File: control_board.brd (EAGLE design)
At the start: 90.2 x 72.3 mm, 19 parts

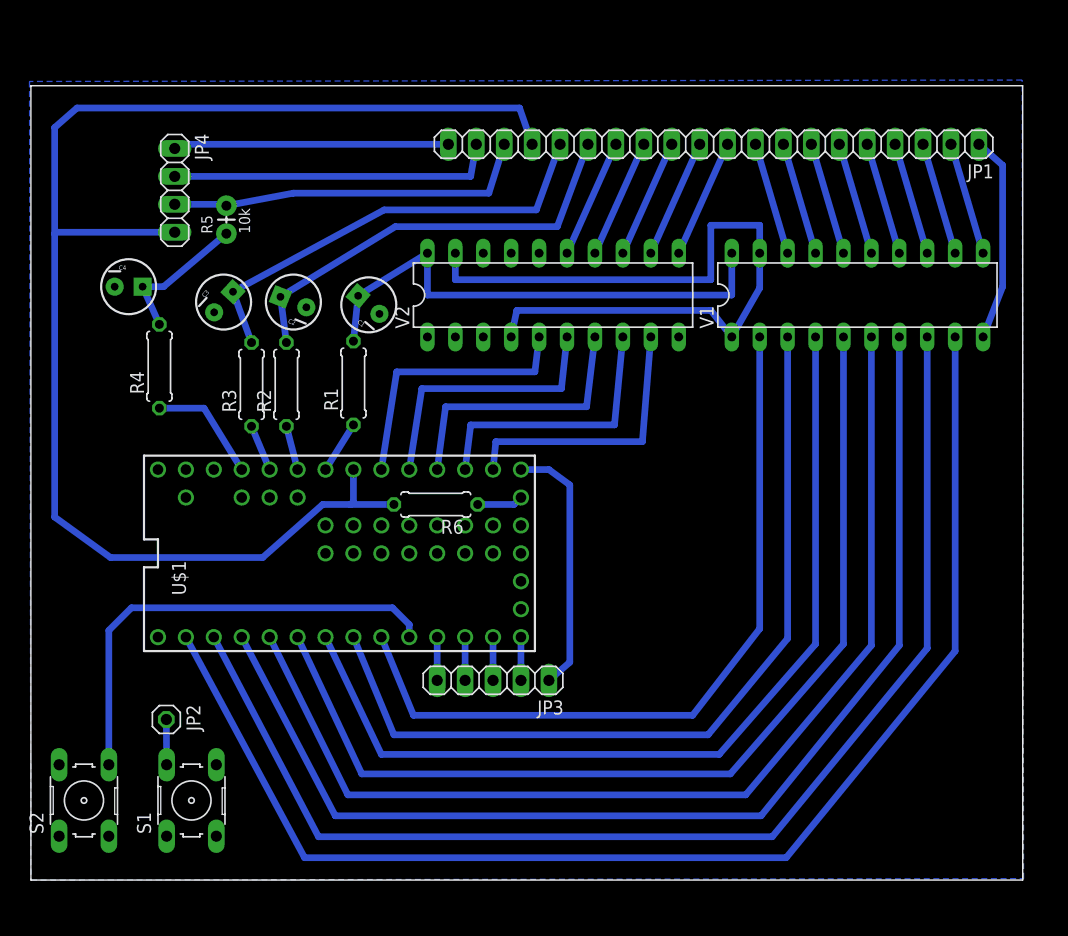
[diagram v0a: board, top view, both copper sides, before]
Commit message: First commit
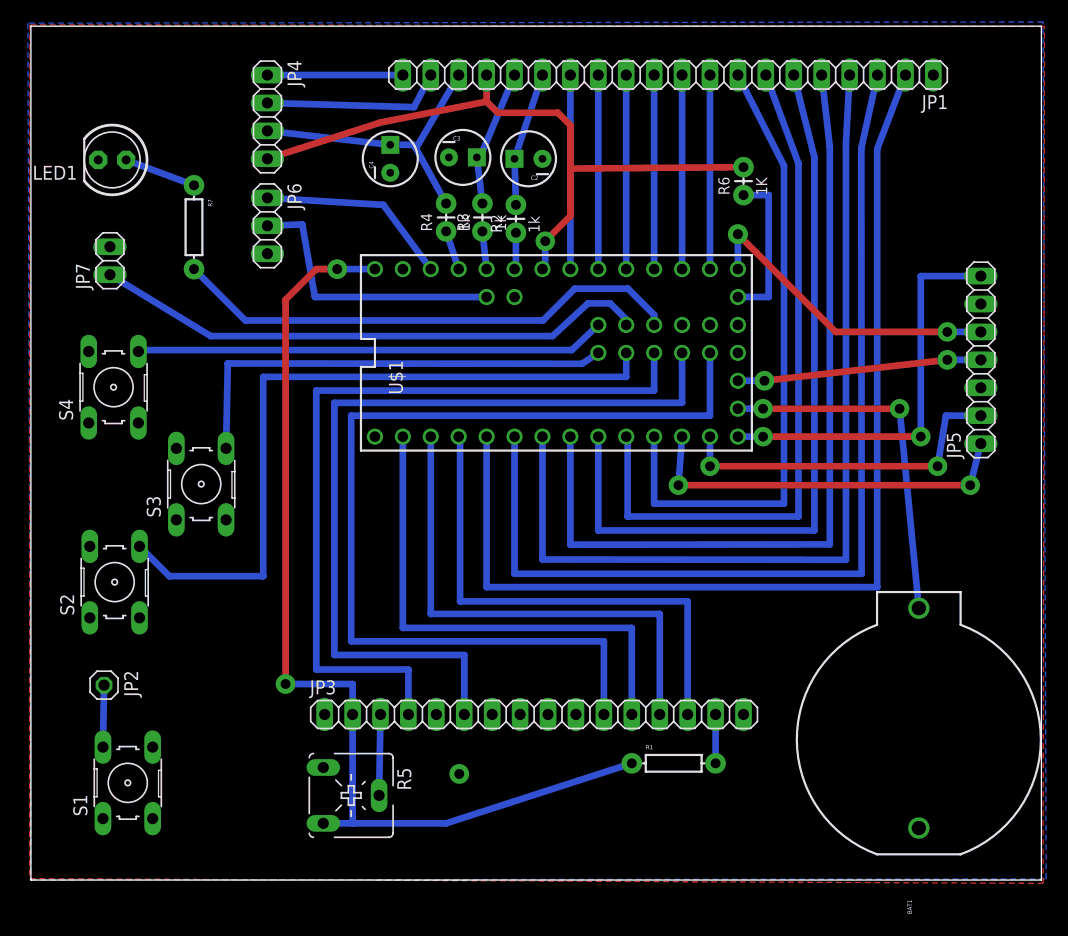
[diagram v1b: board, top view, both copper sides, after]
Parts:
- removed C1: (no value), SparkFun-Capacitors:CPOL-RADIAL-10UF-25V
- removed V1, V2: 74540N, 74ttl-din:DIL20
- added BAT1: (no value), SparkFun-Electromechanical:BATTCOM_20MM_PTH
- added JP5: SD_card, sd_header:1X07
- added JP6: (no value), pinhead:1X03
- added JP7: Buzzer_header, pinhead:1X02
- added LED1: (no value), adafruit:LED5MM
- added R7: (no value), SparkFun-Resistors:AXIAL-0.3EZ
- added S3, S4: (no value), switch-omron:B3F-10XX
- JP3: value (none) -> 16x2_LCD_header; device pinhead:1X05 -> LCD_HEADER:1X16
- R1: value 330 -> (none); device resistor:0207/7 -> SparkFun-Resistors:AXIAL-0.3EZ
- R2, R3, R4: device resistor:0207/7 -> SparkFun-Resistors:AXIAL-0.1
- R5: value 10k -> (none); device SparkFun-Resistors:AXIAL-0.1 -> pot:CA6V
- R6: device rcl:0207/7 -> SparkFun-Resistors:AXIAL-0.1
- U$1: value TEENSY_3.0_ALLPINS -> TEENSY_31_ALLPINS_DIGITAL; device Teensy3.0:TEENSY_3.0_ALLPINS -> Teensy3.0:TEENSY_31_ALLPINS_DIGITAL
- moved R5 52.4 mm to (29.1, 7.70), turned to 270 degrees
- moved R1 45.2 mm to (58.5, 10.6), turned to 0 degrees
- moved R6 39.7 mm to (64.8, 62.3), turned to 90 degrees
- moved R4 28.8 mm to (37.8, 59.0)
- moved U$1 27.8 mm to (49.1, 48.0)
- moved C4 26.5 mm to (32.7, 65.6), turned to 90 degrees
- moved C3 25.4 mm to (39.3, 65.7), turned to 0 degrees
- moved R3 25.2 mm to (41.1, 59.0)
- moved C2 25.0 mm to (45.3, 65.6), turned to 180 degrees
- moved R2 25.0 mm to (44.1, 58.9)
- moved S2 20.1 mm to (7.62, 27.1)
- moved JP4 10.8 mm to (21.5, 69.4)
- moved JP1 7.54 mm to (58.0, 73.2)
- moved JP2 6.47 mm to (6.65, 17.7)
- moved S1 6.01 mm to (8.81, 8.84)
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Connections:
- removed net +UB: C1.1, R1.2, V1.20, V2.20
- removed net AREF: U$1.AREF
- removed net LEVEL_SHIFTER_POWER_PIN: R1.1, U$1.20/A6
- removed net N0: C4.1, R4.2, R5.P$1
- removed net VBAT: U$1.VBAT
- removed net VIN: U$1.VIN
- removed net VUSB: U$1.VUSB
- new net 3.3V: JP5.3V3, JP6.1, U$1.3.3V
- new net N$37: JP7.1, U$1.32
- net 3DS_C_PAD_X: now also R2.P$2; no longer R2.2
- net 3DS_C_PAD_Y: now also R3.P$2; no longer R3.2
- net 3DS_TOUCH_SCREEN_X: now also C4.1, R4.P$2; no longer R5.P$2
- net 3DS_TOUCH_SCREEN_Y: now also R6.P$2, U$1.20/A6; no longer R6.2, U$1.19/A5
- net C_PAD_X_PIN: now also R2.P$1; no longer R2.1
- net C_PAD_Y_PIN: now also R3.P$1; no longer R3.1
- net GND: now also BAT1.2, JP3.GND, JP3.LED-, JP3.RW, JP5.GND, JP5.GND_2, JP6.3, JP7.2, LED1.K, R5.A, S3.2, S4.2; no longer C1.2, U$1.GND1, U$1.GND2, V1.1, V1.10, V1.19, V2.1, V2.10, V2.19, V2.2, V2.3, V2.4
- net N$1: now also JP1.7, U$1.8; no longer JP1.2, V1.11
- net N$10: now also JP3.CONTRAST, R5.S; no longer JP1.12, V2.13
- net N$11: now also JP5.SS, U$1.10; no longer JP1.13, V2.14
- net N$12: now also JP5.MOSI, U$1.11; no longer JP1.14, V2.15
- net N$13: now also JP5.MISO, U$1.12; no longer JP1.10, V2.11
- net N$15: now also JP5.SCK, U$1.13; no longer U$1.14/A0, V2.9
- net N$16: now also JP6.2, U$1.A10; no longer U$1.15/A1, V2.8
- net N$17: now also JP3.D7, U$1.2; no longer U$1.16/A2, V2.7
- net N$18: now also JP3.D6, U$1.1; no longer U$1.17/A3, V2.6
- net N$19: now also JP3.D5; no longer V1.9
- net N$2: now also JP1.8, U$1.9; no longer JP1.3, V1.12
- net N$20: now also JP3.D4, U$1.28; no longer U$1.1, V1.8
- net N$21: now also JP3.E, U$1.27; no longer U$1.2, V1.7
- net N$22: now also JP1.2; no longer V1.6
- net N$23: now also JP1.3; no longer V1.5
- net N$24: now also JP1.4; no longer V1.4
- net N$25: now also JP1.5; no longer V1.3
- net N$26: now also JP1.6; no longer V1.2
- net N$27: now also R6.P$1; no longer R6.1
- net N$28: now also JP3.RS, U$1.26; no longer U$1.18/A4, V2.5
- net N$29: now also BAT1.1, U$1.VBAT; no longer JP3.5, U$1.9
- net N$3: now also JP1.9, U$1.14/A0; no longer JP1.4, V1.13
- net N$30: now also S2.4, U$1.25; no longer JP3.4, U$1.10
- net N$31: now also S3.4, U$1.24; no longer JP3.3, U$1.11
- net N$32: now also S4.4, U$1.33; no longer JP3.2, U$1.12
- net N$33: now also R7.P$2, U$1.31; no longer JP3.1, U$1.13
- net N$36: now also LED1.A, R7.P$1; no longer S2.4, U$1.8
- net N$4: now also JP1.10, U$1.15/A1; no longer JP1.5, V1.14
- net N$5: now also JP1.11, U$1.16/A2; no longer JP1.6, V1.15
- net N$6: now also JP1.12, U$1.17/A3; no longer JP1.7, V1.16
- net N$7: now also JP1.13, U$1.18/A4; no longer JP1.8, V1.17
- net N$8: now also JP1.14, U$1.19/A5; no longer JP1.9, V1.18
- net N$9: now also JP3.LED+, R1.P$2; no longer JP1.11, V2.12
- net TOUCH_SCREEN_X_PIN: now also R4.P$1; no longer R4.1
- net VCC: now also JP3.5V, R1.P$1, R5.E, U$1.VIN; no longer U$1.3.3V, U$1.3.3V1, U$1.3.3V2
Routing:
- net VCC: track 0.00 -> 91.9 mm, vias 0 -> 2
- net GND: track 87.9 -> 0.00 mm, vias 0 -> 1
- net N$19: track 119.5 -> 46.1 mm
- net 3DS_TOUCH_SCREEN_Y: track 130.0 -> 61.6 mm, vias 0 -> 1
- net N$30: track 3.94 -> 65.7 mm
- net N$1: track 10.3 -> 63.5 mm
- net N$37: track 0.00 -> 50.8 mm
- net N$2: track 10.3 -> 57.9 mm
- net N$28: track 24.8 -> 72.0 mm
- net +UB: track 46.9 -> 0.00 mm
- net 3.3V: track 0.00 -> 40.0 mm, vias 0 -> 2
- net N$32: track 3.94 -> 42.8 mm
- net N$31: track 3.94 -> 41.7 mm
- net N$36: track 42.2 -> 6.59 mm
- net N$29: track 3.94 -> 32.9 mm, vias 0 -> 2
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- added copper zone on layer 1, net GND
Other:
- board size 90.2 x 72.3 mm -> 91.9 x 77.7 mm
